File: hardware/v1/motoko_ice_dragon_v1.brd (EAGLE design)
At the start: 100 x 80 mm, 121 parts, among them Q1 8MHz, Q10 20mA/30V, Q11 20mA/30V, Q2 BSS138TOP, Q4 20mA/30V, Q5 20mA/30V, Q6 20mA/30V, Q7 20mA/30V, Q8 20mA/30V, Q9 20mA/30V, U1 MP6540HA, U2 STM32_STM32F722XX, U3 MP6540HA, U4 AP63203, X1 FH12-12S-0.5SH, X2 FH12-12S-0.5SH, X3 52745-0490, X4 52745-0490, X5 52745-0490

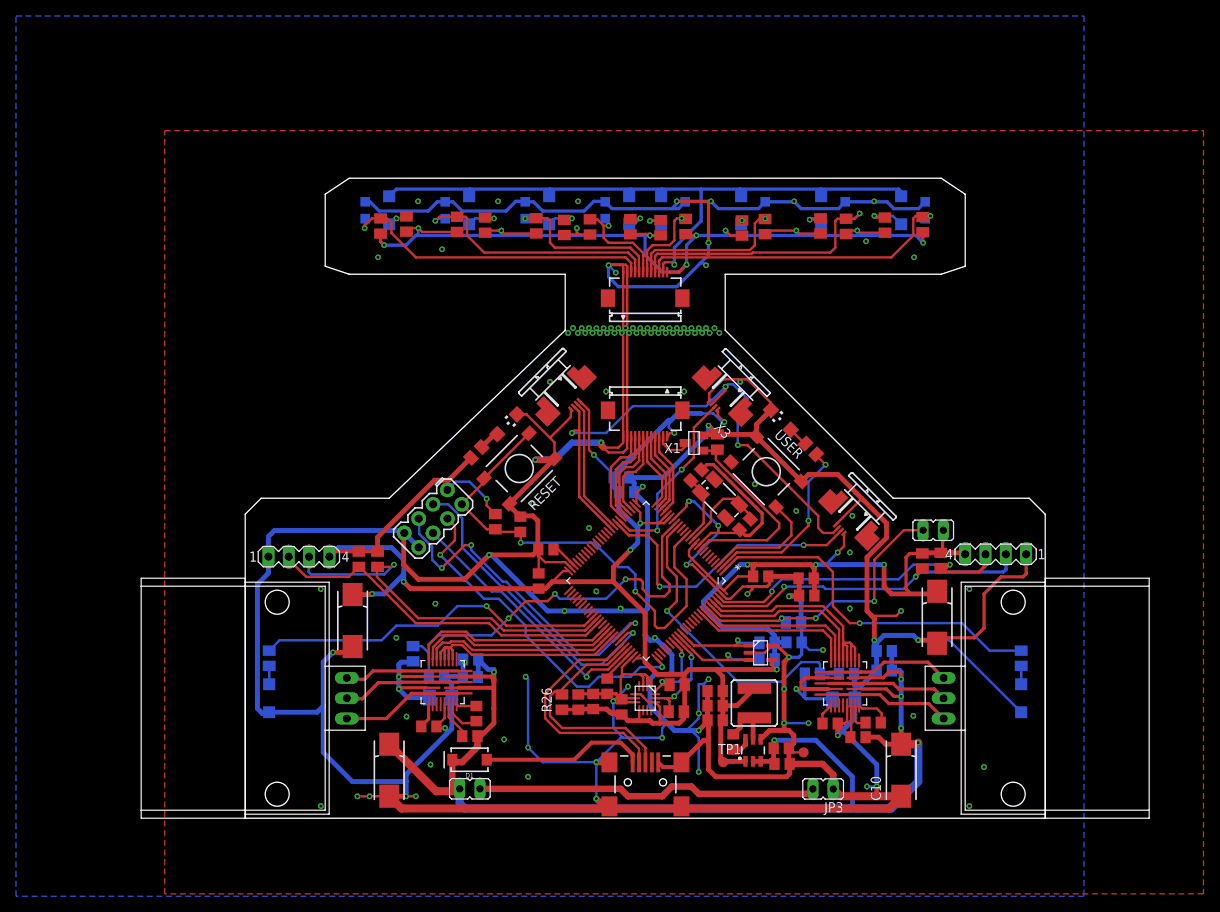
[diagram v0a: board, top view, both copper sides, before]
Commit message: new foc
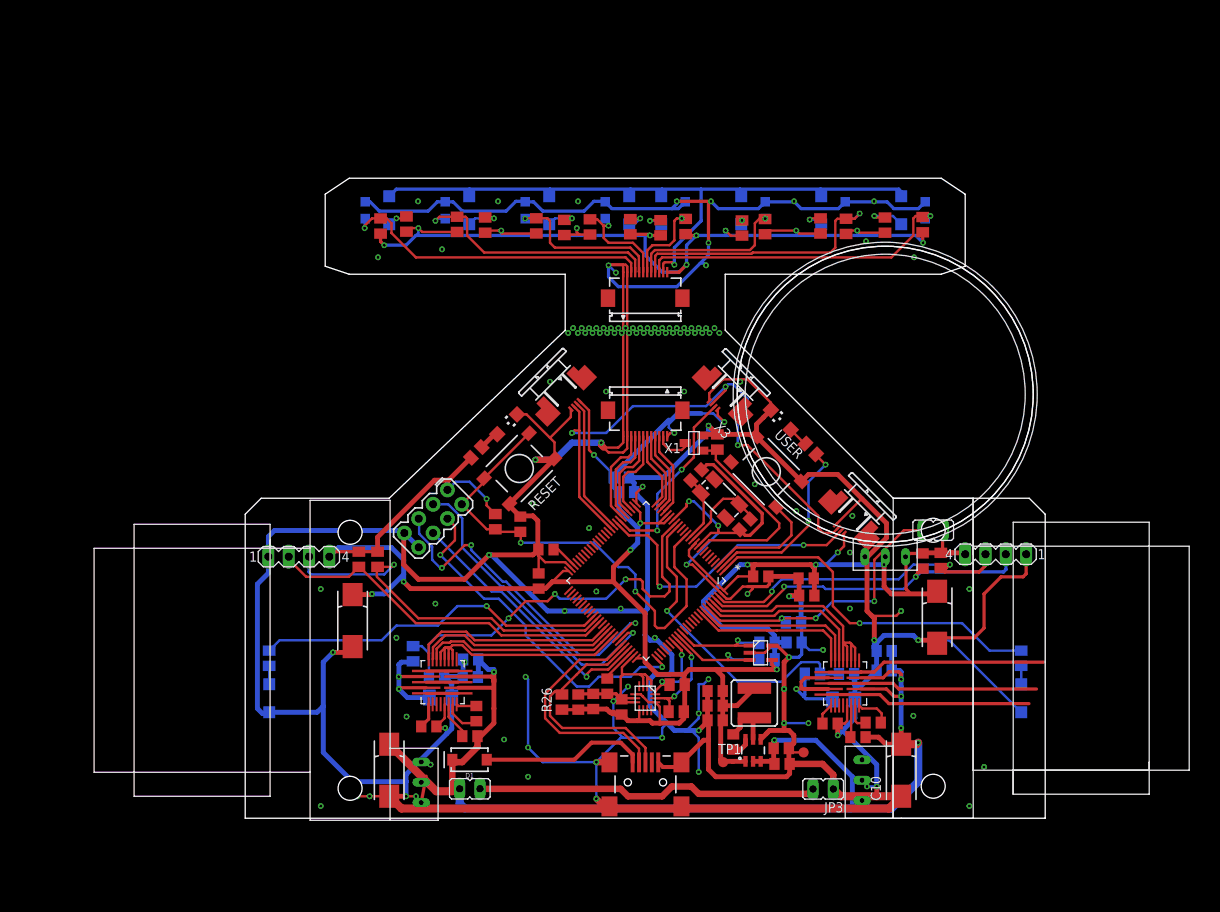
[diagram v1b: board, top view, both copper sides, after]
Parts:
- added U$5: DUCTED_FAN_35MM, my_library:DUCTED_FAN_35MM
- U$1, U$2: value BRUSHLESS_GIMBAL_MOTOR_WHEEL -> BRUSHLESS_MOTOR_WHEEL; device my_library:BRUSHLESS_GIMBAL_MOTOR_WHEEL -> my_library:BRUSHLESS_MOTOR_WHEEL
- moved U$2 14.9 mm to (86.0, 20.0), flipped to the bottom, turned to 0 degrees
- moved U$1 13.9 mm to (13.1, 19.7)
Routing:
- net R_YA: track 15.7 -> 27.4 mm
- net L_YC: track 15.2 -> 4.01 mm
- net R_YB: track 15.1 -> 26.3 mm
- net L_YB: track 14.8 -> 4.01 mm
- net R_YC: track 15.6 -> 25.5 mm
- net L_YA: track 14.4 -> 7.37 mm
- removed copper zone on layer 1, net GND
- removed copper zone on layer 16, net GND
